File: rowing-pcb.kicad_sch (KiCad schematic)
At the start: 25 parts, among them U1 ESP32-S3-WROOM-1, U2 TP4056, U4 ICM-45686

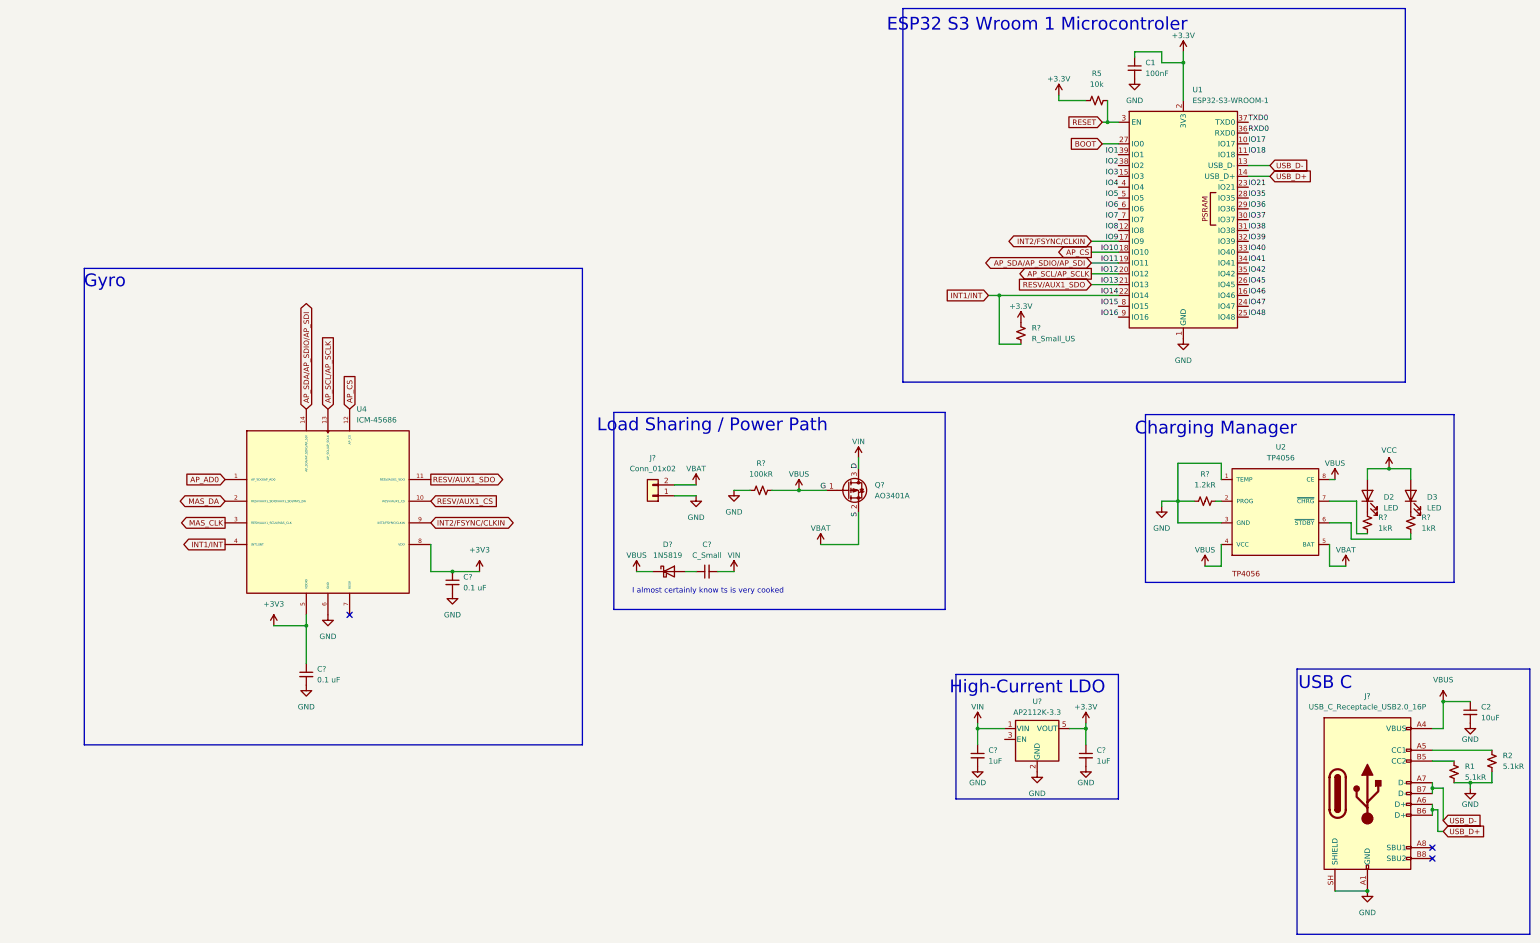
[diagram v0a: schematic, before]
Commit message: new gyro
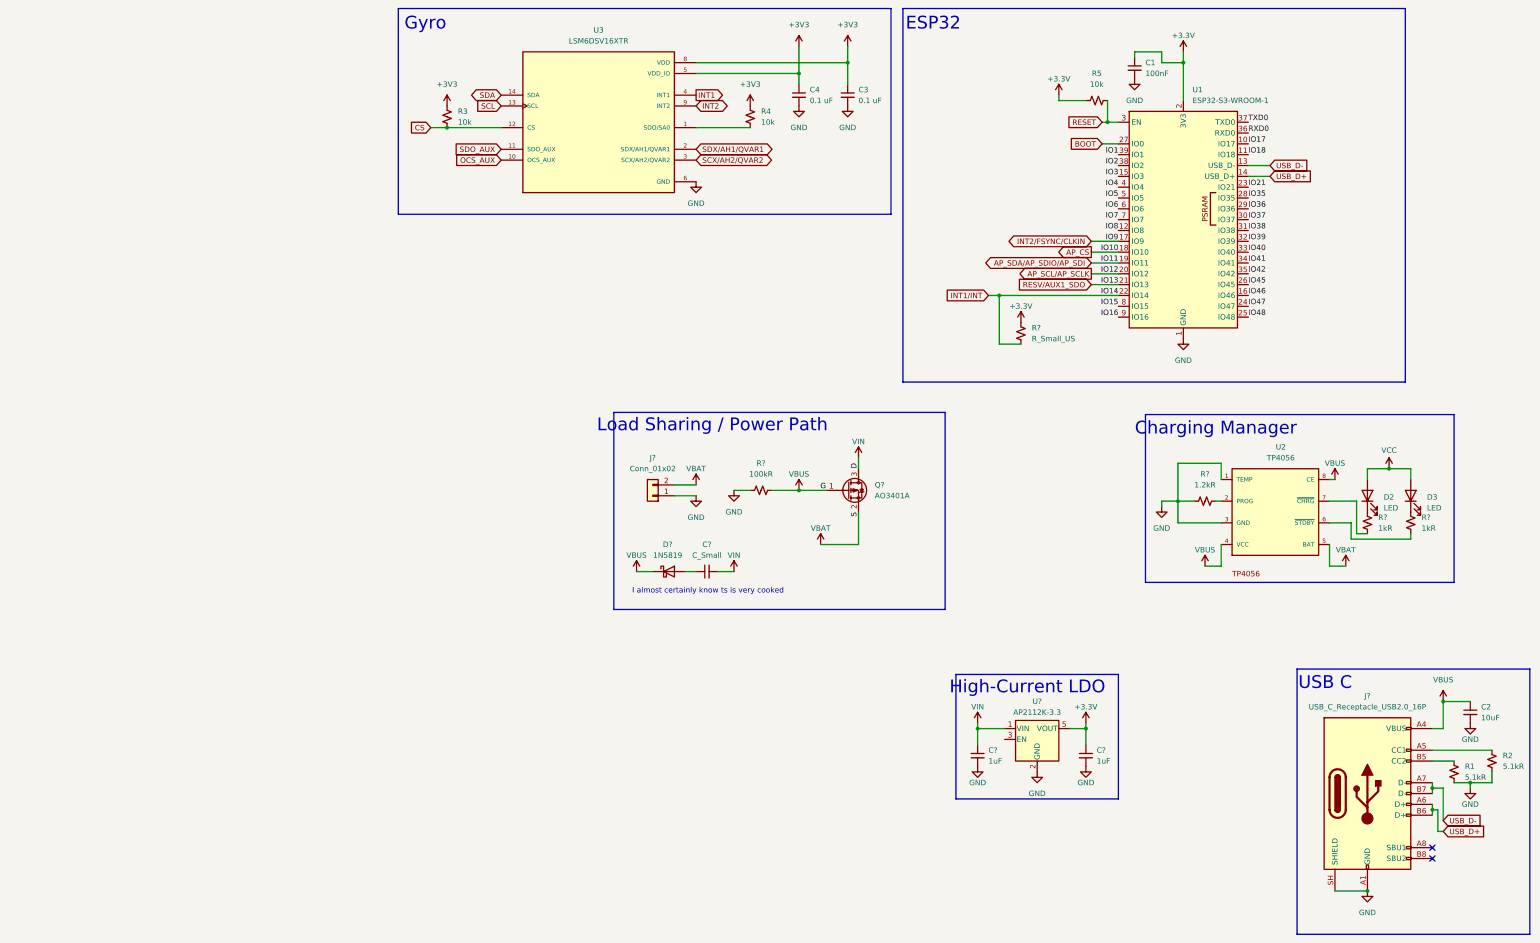
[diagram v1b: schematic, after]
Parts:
- removed C? (x2): 0.1 uF, symbol Device:C_Small
- removed U4: ICM-45686, ICM-45686:IC_ICM-45686, symbol ICM-45686:ICM-45686
- added C3, C4: 0.1 uF, symbol Device:C_Small
- added R3, R4: 10k, symbol Device:R_Small_US
- added U3: LSM6DSV16XTR, LSM6DSV16XTR:XDCR_LSM6DSV16XTR, symbol LSM6DSV16XTR:LSM6DSV16XTR
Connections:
- net +3V3: now also C3.1, C4.1, R3.2, R4.2, U3.5 (VDD_IO), U3.8 (VDD)
- net GND: now also C3.2, C4.2, U3.6 (GND), U3.7 (GND)
- new net: R4.1, U3.1 (SDO/SA0)
- new net CS: R3.1, U3.12 (CS)
- new net INT1: U3.4 (INT1)
- new net INT2: U3.9 (INT2)
- new net OCS_AUX: U3.10 (OCS_AUX)
- new net SCL: U3.13 (SCL)
- new net SCX/AH2/QVAR2: U3.3 (SCX/AH2/QVAR2)
- new net SDA: U3.14 (SDA)
- new net SDO_AUX: U3.11 (SDO_AUX)
- new net SDX/AH1/QVAR1: U3.2 (SDX/AH1/QVAR1)
- no-connect marks 3 -> 2
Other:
- note added: "ESP32"
- note removed: "ESP32 S3 Wroom 1 Microcontroler"

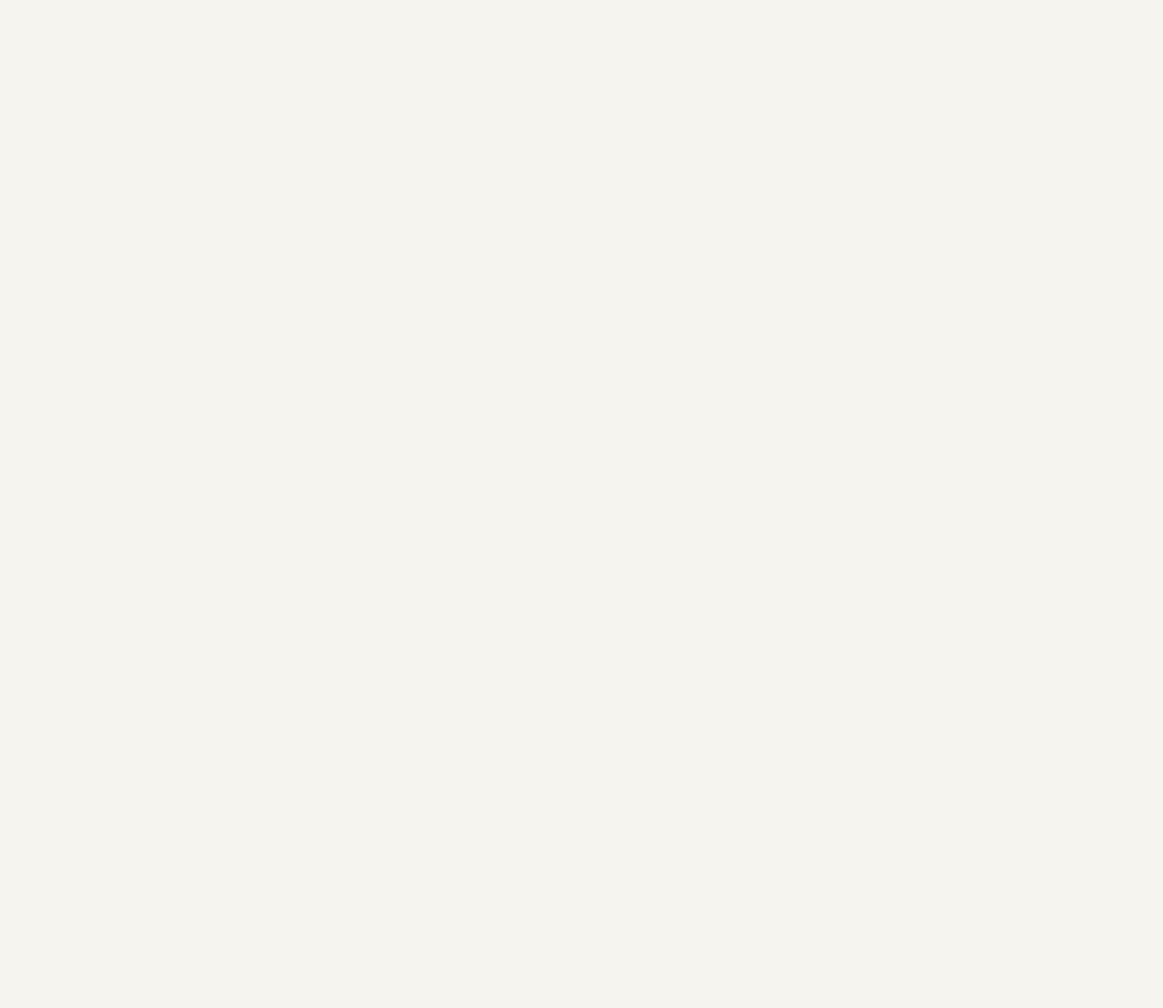
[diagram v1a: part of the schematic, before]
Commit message: added gps
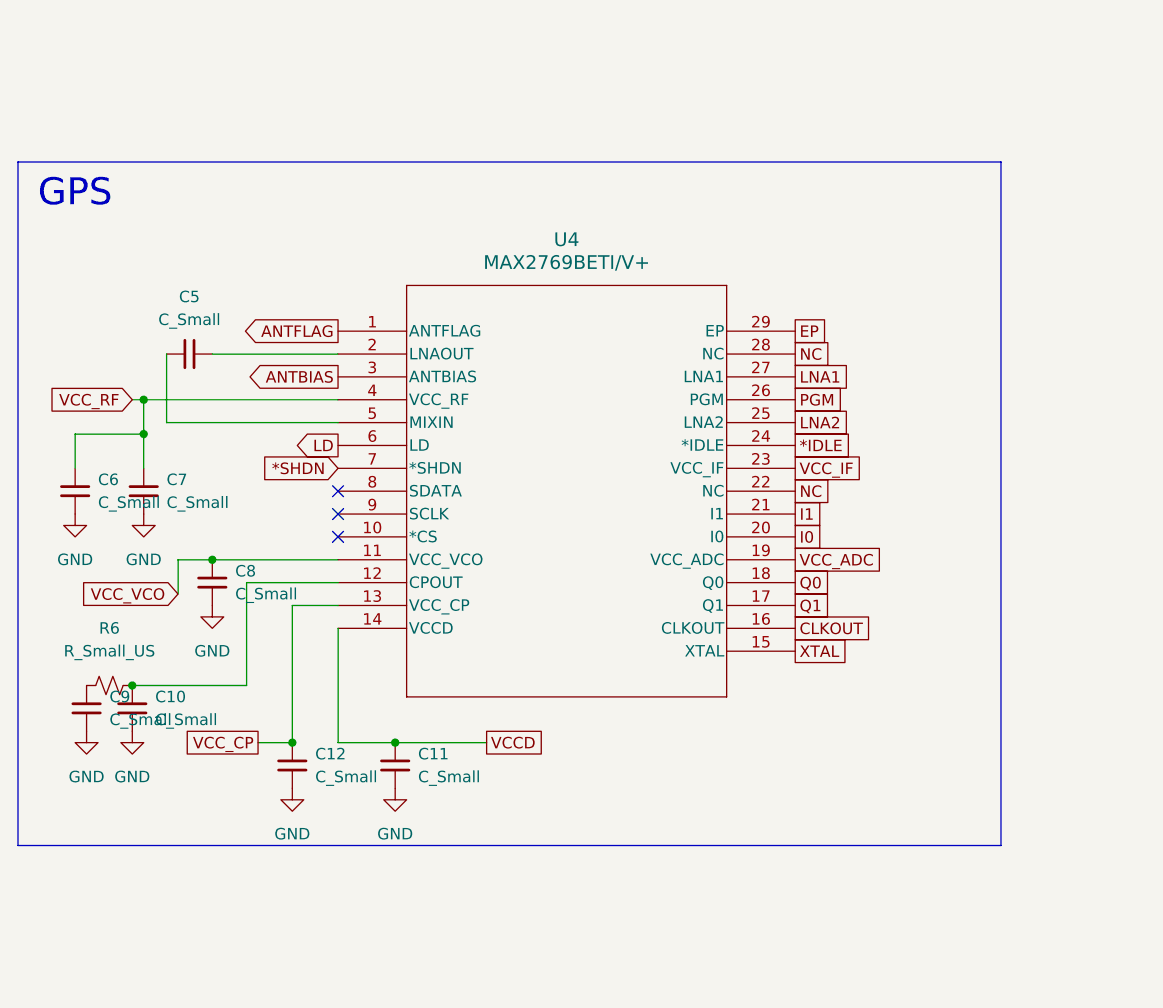
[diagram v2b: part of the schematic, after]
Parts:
- added C10, C11, C12, C5, C6, C7, C8, C9: C_Small, 21-0140_T2855+3_MXM, symbol Device:C_Small
- added R6: R_Small_US, Resistor_THT:R_Array_SIP4, symbol Device:R_Small_US
- added U4: MAX2769BETI/V+, 21-0140_T2855+3_MXM, symbol 2026-10-15_20-01-52:MAX2769BETI_V+
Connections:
- net GND: now also C10.2, C11.2, C12.2, C6.2, C7.2, C8.2, C9.2
- new net: C5.1, U4.2 (LNAOUT)
- new net: C5.2, U4.5 (MIXIN)
- new net: C9.1, R6.1
- new net: C10.1, R6.2, U4.12 (CPOUT)
- new net *IDLE: U4.24 (*IDLE)
- new net *SHDN: U4.7 (*SHDN)
- new net ANTBIAS: U4.3 (ANTBIAS)
- new net ANTFLAG: U4.1 (ANTFLAG)
- new net CLKOUT: U4.16 (CLKOUT)
- new net EP: U4.29 (EP)
- new net I0: U4.20 (I0)
- new net I1: U4.21 (I1)
- new net LD: U4.6 (LD)
- new net LNA1: U4.27 (LNA1)
- new net LNA2: U4.25 (LNA2)
- new net NC: U4.22 (NC), U4.28 (NC)
- new net PGM: U4.26 (PGM)
- new net Q0: U4.18 (Q0)
- new net Q1: U4.17 (Q1)
- new net VCCD: C11.1, U4.14 (VCCD)
- new net VCC_ADC: U4.19 (VCC_ADC)
- new net VCC_CP: C12.1, U4.13 (VCC_CP)
- new net VCC_IF: U4.23 (VCC_IF)
- new net VCC_RF: C6.1, C7.1, U4.4 (VCC_RF)
- new net VCC_VCO: C8.1, U4.11 (VCC_VCO)
- new net XTAL: U4.15 (XTAL)
- no-connect marks 2 -> 5
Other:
- note added: "GPS"
